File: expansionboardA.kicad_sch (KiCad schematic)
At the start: 60 parts, among them J1 DEBUG, J2 USB_A_Stacked, J3 HDMI_A, J4 FAN, P1 USB_C_Plug, U1 MAX3420EECJ, U2 GPIO_U2, U3 AMS1117-3.3, U4 GPIO_U4, U5 MCP3008T-I/SL, U6 CS4344-CZZR, U7 MAX3421EEHJ+T, Y1 Crystal, Y2 Crystal

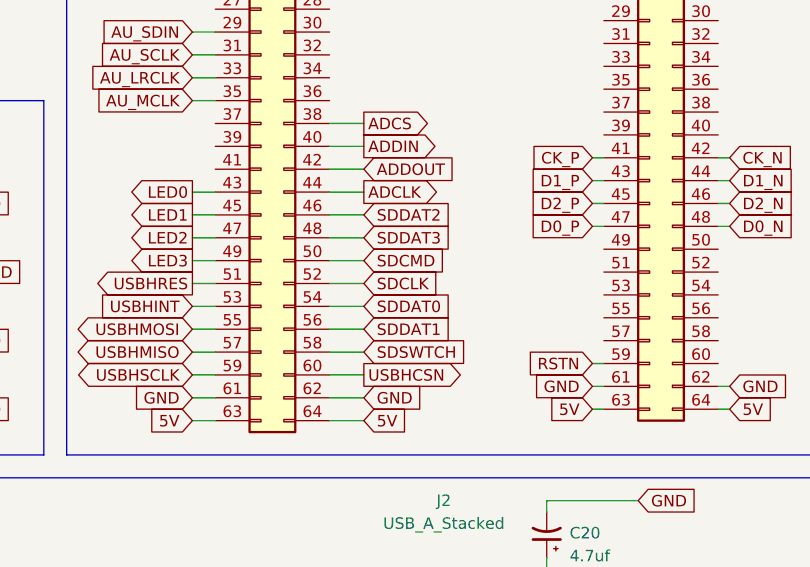
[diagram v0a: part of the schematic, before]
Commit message: Board changes
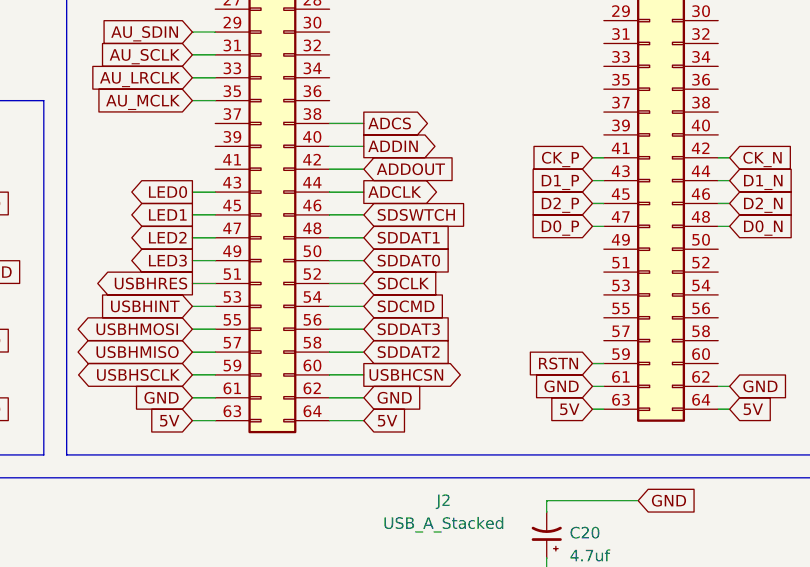
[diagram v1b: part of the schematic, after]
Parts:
- C20, C5: footprint Capacitor_THT:CP_Radial_D4.0mm_P1.50mm -> Capacitor_SMD:CP_Elec_4x5.4
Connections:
- net SDCMD: now also U2.54 (Pin_54); no longer U2.50 (Pin_50)
- net SDDAT0: now also U2.50 (Pin_50); no longer U2.54 (Pin_54)
- net SDDAT1: now also U2.48 (Pin_48); no longer U2.56 (Pin_56)
- net SDDAT2: now also U2.58 (Pin_58); no longer U2.46 (Pin_46)
- net SDDAT3: now also U2.56 (Pin_56); no longer U2.48 (Pin_48)
- net SDSWTCH: now also U2.46 (Pin_46); no longer U2.58 (Pin_58)
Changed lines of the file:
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@@
     (stroke (width 0) (type default))
   )
-  (wire (pts (xy 219.71 139.7) (xy 215.9 139.7))
-    (stroke (width 0) (type default))
-  )
   (wire (pts (xy 200.66 152.4) (xy 203.2 152.4))
     (stroke (width 0) (type default))
@@
     (stroke (width 0) (type default))
   )
+  (wire (pts (xy 215.9 147.32) (xy 219.71 147.32))
+    (stroke (width 0) (type default))
+  )
   (wire (pts (xy 219.71 132.08) (xy 215.9 132.08))
     (stroke (width 0) (type default))
@@
     (stroke (width 0) (type default))
   )
-  (wire (pts (xy 219.71 134.62) (xy 215.9 134.62))
-    (stroke (width 0) (type default))
-  )
   (wire (pts (xy 358.14 214.63) (xy 374.65 214.63))
     (stroke (width 0) (type default))
@@
     (stroke (width 0) (type default))
   )
-  (wire (pts (xy 219.71 144.78) (xy 215.9 144.78))
-    (stroke (width 0) (type default))
-  )
   (wire (pts (xy 388.62 214.63) (xy 386.08 214.63))
     (stroke (width 0) (type default))
@@
     (stroke (width 0) (type default))
   )
-  (wire (pts (xy 361.95 83.82) (xy 361.95 85.09))
+  (wire (pts (xy 215.9 134.62) (xy 219.71 134.62))
     (stroke (width 0) (type default))
   )
-  (wire (pts (xy 219.71 142.24) (xy 215.9 142.24))
+  (wire (pts (xy 361.95 83.82) (xy 361.95 85.09))
     (stroke (width 0) (type default))
   )
@@
     (stroke (width 0) (type default))
   )
-  (wire (pts (xy 278.13 53.34) (xy 278.13 50.8))
+  (wire (pts (xy 215.9 149.86) (xy 219.71 149.86))
     (stroke (width 0) (type default))
   )
-  (wire (pts (xy 245.11 39.37) (xy 255.27 39.37))
+  (wire (pts (xy 278.13 53.34) (xy 278.13 50.8))
     (stroke (width 0) (type default))
   )
-  (wire (pts (xy 219.71 137.16) (xy 215.9 137.16))
+  (wire (pts (xy 245.11 39.37) (xy 255.27 39.37))
     (stroke (width 0) (type default))
   )
@@
     (stroke (width 0) (type default))
   )
+  (wire (pts (xy 215.9 142.24) (xy 219.71 142.24))
+    (stroke (width 0) (type default))
+  )
   (wire (pts (xy 217.17 88.9) (xy 215.9 88.9))
     (stroke (width 0) (type default))
@@
     (stroke (width 0) (type default))
   )
-  (wire (pts (xy 219.71 149.86) (xy 215.9 149.86))
-    (stroke (width 0) (type default))
-  )
   (wire (pts (xy 364.49 194.31) (xy 374.65 194.31))
     (stroke (width 0) (type default))
@@
     (stroke (width 0) (type default))
   )
+  (wire (pts (xy 215.9 137.16) (xy 219.71 137.16))
+    (stroke (width 0) (type default))
+  )
   (wire (pts (xy 308.61 158.75) (xy 308.61 156.21))
     (stroke (width 0) (type default))
@@
     (stroke (width 0) (type default))
   )
-  (wire (pts (xy 219.71 147.32) (xy 215.9 147.32))
-    (stroke (width 0) (type default))
-  )
   (wire (pts (xy 334.01 49.53) (xy 334.01 57.15))
     (stroke (width 0) (type default))
@@
     (stroke (width 0) (type default))
   )
+  (wire (pts (xy 215.9 139.7) (xy 219.71 139.7))
+    (stroke (width 0) (type default))
+  )
   (wire (pts (xy 308.61 148.59) (xy 308.61 146.05))
     (stroke (width 0) (type default))
@@
     (stroke (width 0) (type default))
   )
+  (wire (pts (xy 215.9 144.78) (xy 219.71 144.78))
+    (stroke (width 0) (type default))
+  )
   (wire (pts (xy 149.86 224.79) (xy 153.67 224.79))
     (stroke (width 0) (type default))
@@
     )
   )
-  (global_label "SDDAT2" (shape input) (at 219.71 134.62 0) (fields_autoplaced)
+  (global_label "SDDAT2" (shape input) (at 219.71 149.86 0) (fields_autoplaced)
     (effects (font (size 1.27 1.27)) (justify left))
-    (property "Intersheetrefs" "${INTERSHEET_REFS}" (at 229.631 134.62 0)
+    (property "Intersheetrefs" "${INTERSHEET_REFS}" (at 229.631 149.86 0)
       (effects (font (size 1.27 1.27)) (justify left) hide)
     )
@@
     )
   )
-  (global_label "SDSWTCH" (shape input) (at 219.71 149.86 0) (fields_autoplaced)
+  (global_label "SDSWTCH" (shape input) (at 219.71 134.62 0) (fields_autoplaced)
     (effects (font (size 1.27 1.27)) (justify left))
-    (property "Intersheetrefs" "${INTERSHEET_REFS}" (at 231.3243 149.86 0)
+    (property "Intersheetrefs" "${INTERSHEET_REFS}" (at 231.3243 134.62 0)
       (effects (font (size 1.27 1.27)) (justify left) hide)
     )
@@
     )
   )
-  (global_label "SDCMD" (shape input) (at 219.71 139.7 0) (fields_autoplaced)
+  (global_label "SDCMD" (shape input) (at 219.71 144.78 0) (fields_autoplaced)
     (effects (font (size 1.27 1.27)) (justify left))
-    (property "Intersheetrefs" "${INTERSHEET_REFS}" (at 229.0867 139.7 0)
+    (property "Intersheetrefs" "${INTERSHEET_REFS}" (at 229.0867 144.78 0)
       (effects (font (size 1.27 1.27)) (justify left) hide)
     )
@@
     )
   )
-  (global_label "SDDAT1" (shape input) (at 219.71 147.32 0) (fields_autoplaced)
+  (global_label "SDDAT1" (shape input) (at 219.71 137.16 0) (fields_autoplaced)
     (effects (font (size 1.27 1.27)) (justify left))
-    (property "Intersheetrefs" "${INTERSHEET_REFS}" (at 229.631 147.32 0)
+    (property "Intersheetrefs" "${INTERSHEET_REFS}" (at 229.631 137.16 0)
       (effects (font (size 1.27 1.27)) (justify left) hide)
     )
@@
     )
   )
-  (global_label "SDDAT3" (shape input) (at 219.71 137.16 0) (fields_autoplaced)
+  (global_label "SDDAT3" (shape input) (at 219.71 147.32 0) (fields_autoplaced)
     (effects (font (size 1.27 1.27)) (justify left))
-    (property "Intersheetrefs" "${INTERSHEET_REFS}" (at 229.631 137.16 0)
+    (property "Intersheetrefs" "${INTERSHEET_REFS}" (at 229.631 147.32 0)
       (effects (font (size 1.27 1.27)) (justify left) hide)
     )
@@
     )
   )
-  (global_label "SDDAT0" (shape input) (at 219.71 144.78 0) (fields_autoplaced)
+  (global_label "SDDAT0" (shape input) (at 219.71 139.7 0) (fields_autoplaced)
     (effects (font (size 1.27 1.27)) (justify left))
-    (property "Intersheetrefs" "${INTERSHEET_REFS}" (at 229.631 144.78 0)
+    (property "Intersheetrefs" "${INTERSHEET_REFS}" (at 229.631 139.7 0)
       (effects (font (size 1.27 1.27)) (justify left) hide)
     )
@@
       (effects (font (size 1.27 1.27)) (justify right))
     )
-    (property "Footprint" "Capacitor_THT:CP_Radial_D4.0mm_P1.50mm" (at 287.02 156.21 0)
+    (property "Footprint" "Capacitor_SMD:CP_Elec_4x5.4" (at 287.02 156.21 0)
       (effects (font (size 1.27 1.27)) hide)
     )
@@
       (effects (font (size 1.27 1.27)) (justify right))
     )
-    (property "Footprint" "Capacitor_THT:CP_Radial_D4.0mm_P1.50mm" (at 240.03 170.18 0)
+    (property "Footprint" "Capacitor_SMD:CP_Elec_4x5.4" (at 240.03 170.18 0)
       (effects (font (size 1.27 1.27)) hide)
     )
